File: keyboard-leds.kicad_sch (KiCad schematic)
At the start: 53 parts, among them J1 USB_C_Receptacle_USB2.0_16P, J2 Conn_01x05, J4 Conn_01x03, J5 USB_C_Receptacle_USB2.0_16P, U1 RP2040, U2 W25Q128JVS, U3 XC6206PxxxMR-Regulator_Linear, U4 TFT_320x240, U5 TUSB320, U6 SN74AHCT1G125DBVR, U7 SRV05-4, U8 TPS2121RUXT, Y1 Crystal_GND24

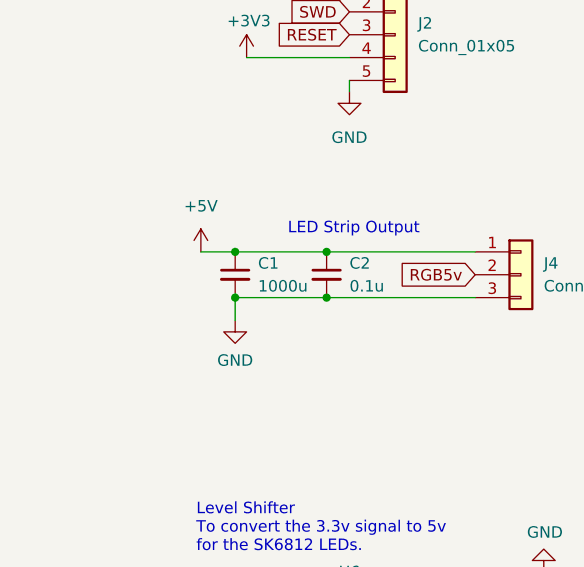
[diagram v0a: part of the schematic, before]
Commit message: Updates
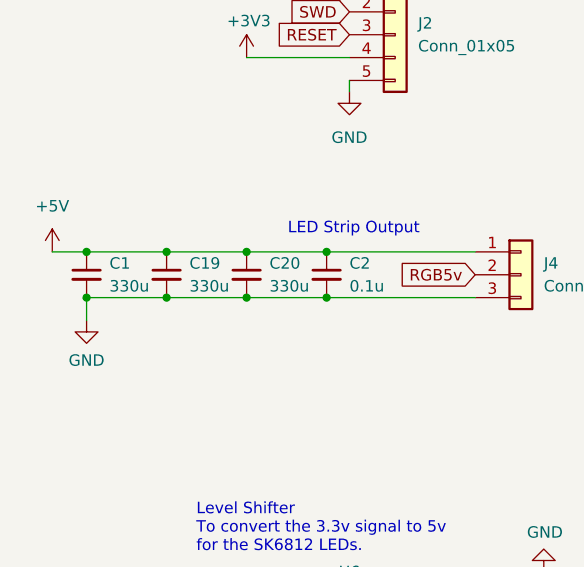
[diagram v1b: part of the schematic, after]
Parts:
- added C19, C20: 330u, Capacitor_Tantalum_SMD:CP_EIA-7343-31_Kemet-D, symbol Device:C_Small
- C1: value 1000u -> 330u; footprint Capacitor_SMD:C_0603_1608Metric -> Capacitor_Tantalum_SMD:CP_EIA-7343-31_Kemet-D
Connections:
- net +5V: now also C19.1, C20.1
- net GND: now also C19.2, C20.2
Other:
- moved on the sheet: C1
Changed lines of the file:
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@@
 	)
 	(junction
-		(at 40.64 204.47)
+		(at 24.13 204.47)
 		(diameter 0)
 		(color 0 0 0 0)
@@
 	)
 	(junction
-		(at 40.64 209.55)
+		(at 33.02 209.55)
+		(diameter 0)
+		(color 0 0 0 0)
+	)
+	(junction
+		(at 24.13 209.55)
 		(diameter 0)
 		(color 0 0 0 0)
@@
 	)
 	(junction
+		(at 41.91 204.47)
+		(diameter 0)
+		(color 0 0 0 0)
+	)
+	(junction
 		(at 208.28 138.43)
 		(diameter 0)
@@
 	)
 	(junction
+		(at 41.91 209.55)
+		(diameter 0)
+		(color 0 0 0 0)
+	)
+	(junction
 		(at 116.205 48.26)
 		(diameter 0)
@@
 	)
 	(junction
+		(at 33.02 204.47)
+		(diameter 0)
+		(color 0 0 0 0)
+	)
+	(junction
 		(at 210.82 135.89)
 		(diameter 0)
@@
 	(wire
 		(pts
+			(xy 33.02 209.55) (xy 41.91 209.55)
+		)
+		(stroke
+			(width 0)
+			(type default)
+		)
+	)
+	(wire
+		(pts
 			(xy 350.52 220.98) (xy 356.235 220.98)
 		)
@@
 	(wire
 		(pts
-			(xy 40.64 209.55) (xy 50.8 209.55)
+			(xy 24.13 209.55) (xy 33.02 209.55)
 		)
 		(stroke
@@
 	(wire
 		(pts
+			(xy 41.91 209.55) (xy 50.8 209.55)
+		)
+		(stroke
+			(width 0)
+			(type default)
+		)
+	)
+	(wire
+		(pts
 			(xy 327.025 39.37) (xy 327.025 38.1)
 		)
@@
 	(wire
 		(pts
+			(xy 33.02 204.47) (xy 41.91 204.47)
+		)
+		(stroke
+			(width 0)
+			(type default)
+		)
+	)
+	(wire
+		(pts
 			(xy 323.85 40.64) (xy 327.025 40.64)
 		)
@@
 	(wire
 		(pts
-			(xy 40.64 204.47) (xy 50.8 204.47)
+			(xy 24.13 204.47) (xy 33.02 204.47)
 		)
 		(stroke
@@
 	(wire
 		(pts
+			(xy 41.91 204.47) (xy 50.8 204.47)
+		)
+		(stroke
+			(width 0)
+			(type default)
+		)
+	)
+	(wire
+		(pts
 			(xy 146.685 30.48) (xy 157.48 30.48)
 		)
@@
 	(wire
 		(pts
-			(xy 40.64 212.09) (xy 40.64 209.55)
+			(xy 24.13 212.09) (xy 24.13 209.55)
 		)
 		(stroke
@@
 	(wire
 		(pts
-			(xy 36.83 204.47) (xy 40.64 204.47)
+			(xy 20.32 204.47) (xy 24.13 204.47)
 		)
 		(stroke
@@
 	(symbol
 		(lib_id "power:+5V")
-		(at 36.83 204.47 0)
+		(at 20.32 204.47 0)
 		(unit 1)
 		(exclude_from_sim no)
@@
 		(fields_autoplaced yes)
 		(property "Reference" "#PWR042"
-			(at 36.83 208.28 0)
+			(at 20.32 208.28 0)
 			(effects
 				(font
@@
 		)
 		(property "Value" "+5V"
-			(at 36.83 199.39 0)
+			(at 20.32 199.39 0)
 			(effects
 				(font
@@
 		)
 		(property "Footprint" ""
-			(at 36.83 204.47 0)
+			(at 20.32 204.47 0)
 			(effects
 				(font
@@
 		)
 		(property "Datasheet" ""
-			(at 36.83 204.47 0)
+			(at 20.32 204.47 0)
 			(effects
 				(font
@@
 		)
 		(property "Description" ""
-			(at 36.83 204.47 0)
+			(at 20.32 204.47 0)
 			(effects
 				(font
@@
 	)
 	(symbol
+		(lib_id "Device:C_Small")
+		(at 33.02 207.01 0)
+		(unit 1)
+		(exclude_from_sim no)
+		(in_bom yes)
+		(on_board yes)
+		(dnp no)
+		(fields_autoplaced yes)
+		(property "Reference" "C19"
+			(at 35.56 205.7462 0)
+			(effects
+				(font
+					(size 1.27 1.27)
+				)
+				(justify left)
+			)
+		)
+		(property "Value" "330u"
+			(at 35.56 208.2862 0)
+			(effects
+				(font
+					(size 1.27 1.27)
+				)
+				(justify left)
+			)
+		)
+		(property "Footprint" "Capacitor_Tantalum_SMD:CP_EIA-7343-31_Kemet-D"
+			(at 33.02 207.01 0)
+			(effects
+				(font
+					(size 1.27 1.27)
+				)
+				(hide yes)
+			)
+		)
+		(property "Datasheet" "~"
+			(at 33.02 207.01 0)
+			(effects
+				(font
+					(size 1.27 1.27)
+				)
+				(hide yes)
+			)
+		)
+		(property "Description" ""
+			(at 33.02 207.01 0)
+			(effects
+				(font
+					(size 1.27 1.27)
+				)
+			)
+		)
+		(pin "1"
+		)
+		(pin "2"
+		)
+		(instances
+			(project "keyboard-leds"
+				(path "/581083f2-de44-4398-88e5-c2c4bedbc4f3"
+					(reference "C19")
+					(unit 1)
+				)
+			)
+		)
+	)
+	(symbol
 		(lib_id "power:GND")
 		(at 356.87 215.9 0)
@@
 	(symbol
 		(lib_id "power:GND")
-		(at 40.64 212.09 0)
+		(at 24.13 212.09 0)
 		(mirror y)
 		(unit 1)
@@
 		(dnp no)
 		(property "Reference" "#PWR034"
-			(at 40.64 218.44 0)
+			(at 24.13 218.44 0)
 			(effects
 				(font
@@
 		)
 		(property "Value" "GND"
-			(at 40.64 216.535 0)
+			(at 24.13 216.535 0)
 			(effects
 				(font
@@
 		)
 		(property "Footprint" ""
-			(at 40.64 212.09 0)
+			(at 24.13 212.09 0)
 			(effects
 				(font
@@
 		)
 		(property "Datasheet" ""
-			(at 40.64 212.09 0)
+			(at 24.13 212.09 0)
 			(effects
 				(font
@@
 		)
 		(property "Description" ""
-			(at 40.64 212.09 0)
+			(at 24.13 212.09 0)
 			(effects
 				(font
@@
 	(symbol
 		(lib_id "Device:C_Small")
-		(at 40.64 207.01 0)
+		(at 24.13 207.01 0)
 		(unit 1)
 		(exclude_from_sim no)
@@
 		(fields_autoplaced yes)
 		(property "Reference" "C1"
-			(at 43.18 205.7462 0)
+			(at 26.67 205.7462 0)
 			(effects
 				(font
@@
 			)
 		)
-		(property "Value" "1000u"
-			(at 43.18 208.2862 0)
+		(property "Value" "330u"
+			(at 26.67 208.2862 0)
 			(effects
 				(font
@@
 			)
 		)
-		(property "Footprint" "Capacitor_SMD:C_0603_1608Metric"
-			(at 40.64 207.01 0)
+		(property "Footprint" "Capacitor_Tantalum_SMD:CP_EIA-7343-31_Kemet-D"
+			(at 24.13 207.01 0)
 			(effects
 				(font
@@
 		)
 		(property "Datasheet" "~"
-			(at 40.64 207.01 0)
+			(at 24.13 207.01 0)
 			(effects
 				(font
@@
 		)
 		(property "Description" ""
-			(at 40.64 207.01 0)
+			(at 24.13 207.01 0)
 			(effects
 				(font
@@
 					(unit 1)
 				)
+			)
+		)
+	)
+	(symbol
+		(lib_id "Device:C_Small")
+		(at 41.91 207.01 0)
+		(unit 1)
+		(exclude_from_sim no)
+		(in_bom yes)
+		(on_board yes)
+		(dnp no)
+		(fields_autoplaced yes)
+		(property "Reference" "C20"
+			(at 44.45 205.7462 0)
+			(effects
+				(font
+					(size 1.27 1.27)
+				)
+				(justify left)
+			)
+		)
+		(property "Value" "330u"
+			(at 44.45 208.2862 0)
+			(effects
+				(font
+					(size 1.27 1.27)
+				)
+				(justify left)
+			)
+		)
+		(property "Footprint" "Capacitor_Tantalum_SMD:CP_EIA-7343-31_Kemet-D"
+			(at 41.91 207.01 0)
+			(effects
+				(font
+					(size 1.27 1.27)
+				)
+				(hide yes)
+			)
+		)
+		(property "Datasheet" "~"
+			(at 41.91 207.01 0)
+			(effects
+				(font
+					(size 1.27 1.27)
+				)
+				(hide yes)
+			)
+		)
+		(property "Description" ""
+			(at 41.91 207.01 0)
+			(effects
+				(font
+					(size 1.27 1.27)
+				)
+			)
+		)
+		(pin "1"
+		)
+		(pin "2"
+		)
+		(instances
+			(project "keyboard-leds"
+				(path "/581083f2-de44-4398-88e5-c2c4bedbc4f3"
+					(reference "C20")
+					(unit 1)
+				)
